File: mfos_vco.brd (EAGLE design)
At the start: 100 x 81.5 mm, 60 parts, among them IC1 TL072P, IC2 TL072P, IC3 TL072P, T1 2N3904, T2 2N3904, U1 POWER, U2 2N5457

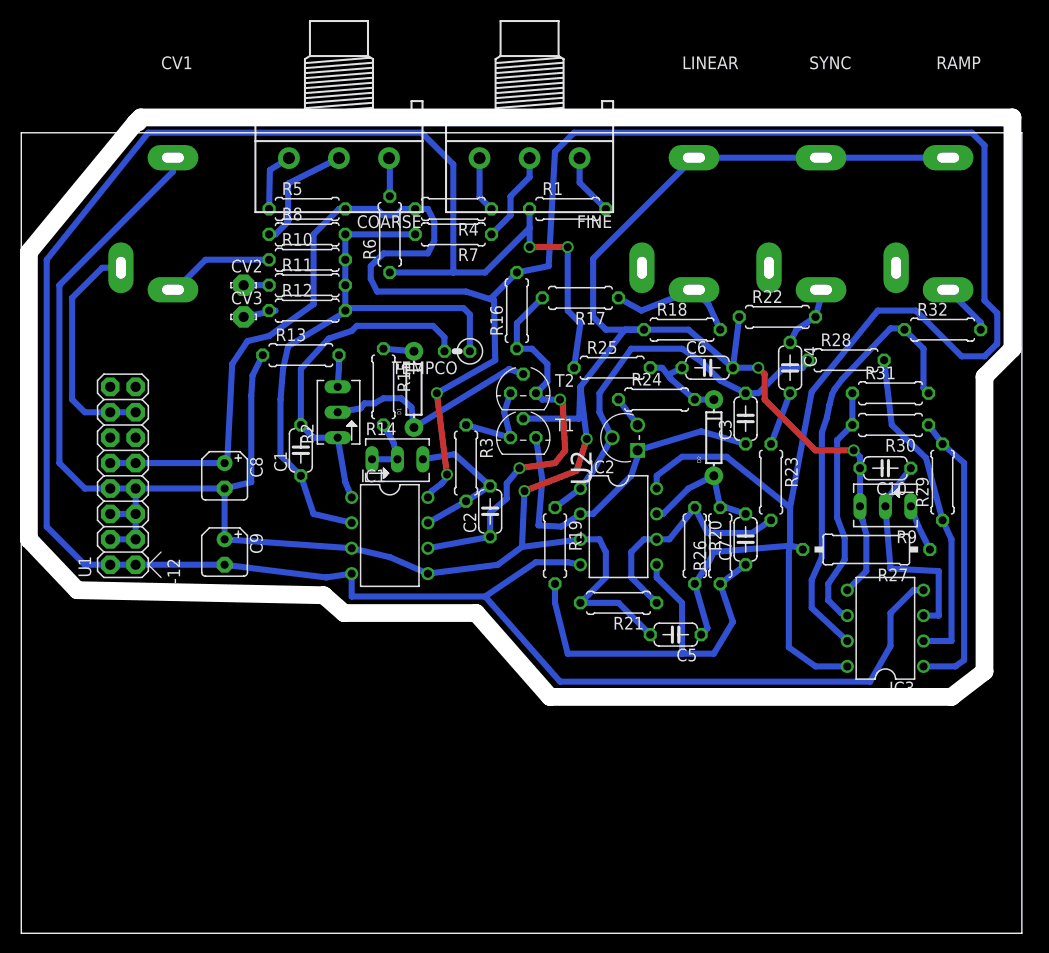
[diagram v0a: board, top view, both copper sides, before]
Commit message: ready to try lm394
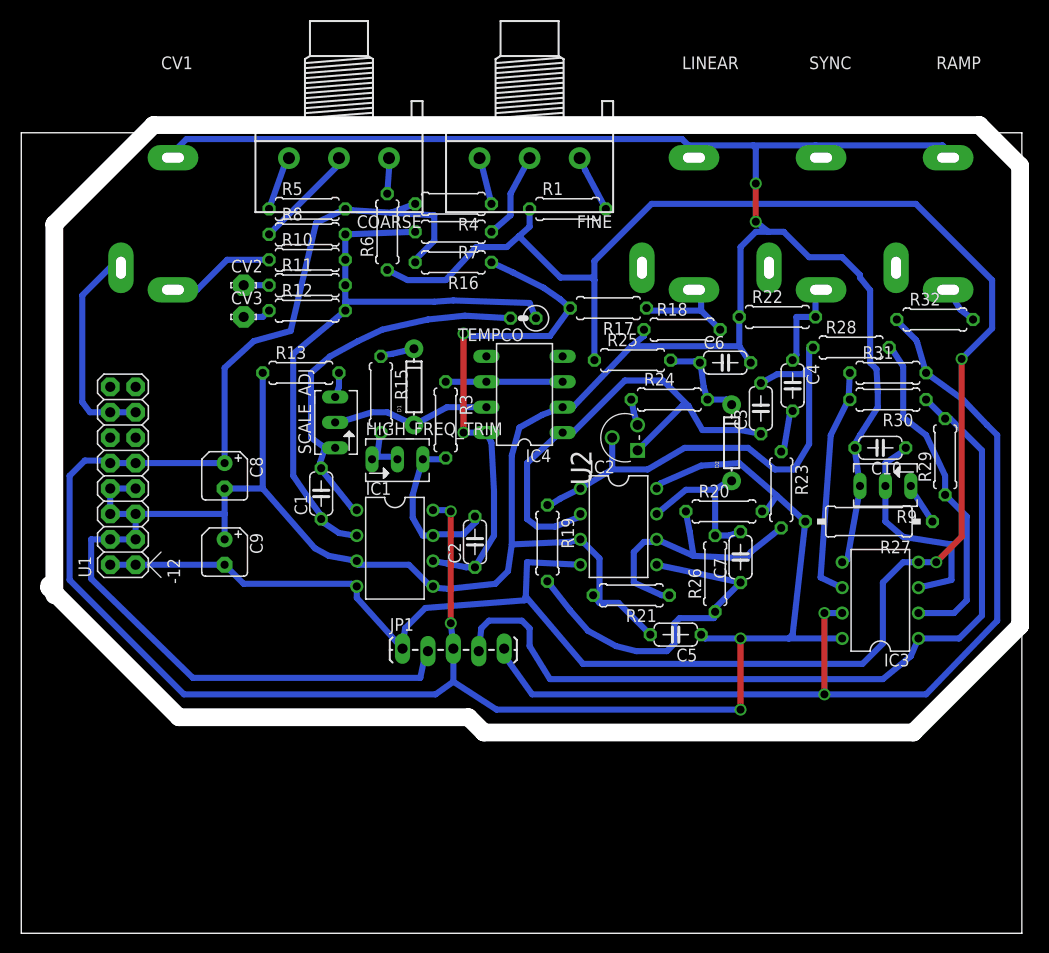
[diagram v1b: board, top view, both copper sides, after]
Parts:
- removed R2: 100R, pot:B64Y
- removed T1, T2: 2N3904, transistor:TO92
- added IC4: LM394N, synthdiy:DIL08
- added JP1: (no value), SparkFun-Connectors:1X05_LOCK_LONGPADS
- added SCALE_ADJ: 100R, pot:B64Y
- moved R16 7.98 mm to (43.2, 67.1), turned to 180 degrees
- moved TEMPCO 7.38 mm to (50.2, 61.5)
- moved R3 4.77 mm to (42.4, 51.3)
- moved C1 4.77 mm to (30.0, 43.9)
- moved R20 4.50 mm to (70.2, 42.2), turned to 0 degrees
- moved C2 3.41 mm to (45.3, 39.1)
- moved R17 2.97 mm to (58.7, 62.5)
- moved IC3 2.84 mm to (85.9, 33.3)
- moved R26 2.84 mm to (69.3, 35.9)
- moved R27 2.81 mm to (84.7, 41.1)
- moved R30 2.55 mm to (86.6, 53.3)
- moved R29 2.55 mm to (92.3, 47.6)
- moved R25 2.17 mm to (61.1, 57.3)
- moved C10 2.09 mm to (85.9, 48.5)
- moved R31 2.05 mm to (86.6, 56.0)
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- renumbered R14 to HIGH_FREQ_TRIM
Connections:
- net +12V: now also JP1.3
- net -12V: now also JP1.1
- net GND: now also IC4.2, JP1.2; no longer T1.2
- net N$12: now also IC4.3, IC4.6; no longer T1.3, T2.3
- net N$13: now also IC4.8; no longer T2.1
- net N$23: now also IC4.1; no longer T1.1
- net N$33: now also JP1.4
- net N$35: now also JP1.5
- net N$7: now also SCALE_ADJ.A; no longer R2.A
- net N$8: now also IC4.7, SCALE_ADJ.S; no longer R2.S, T2.2
- net N$9: now also SCALE_ADJ.E; no longer R2.E
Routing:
- net GND: track 274.4 -> 332.1 mm, vias 4 -> 2
- net +12V: track 277.0 -> 220.4 mm, vias 2 -> 4
- net N$35: track 44.2 -> 99.2 mm, vias 0 -> 2
- net N$33: track 29.2 -> 83.9 mm
- net N$23: track 34.0 -> 48.3 mm
- net N$13: track 40.7 -> 51.8 mm
- net -12V: track 233.9 -> 222.9 mm
- net N$21: track 40.0 -> 48.8 mm
- net N$22: track 42.6 -> 35.2 mm
- net N$8: track 22.8 -> 16.0 mm
- net N$9: track 33.9 -> 38.3 mm
- net N$26: track 24.1 -> 28.2 mm
- net N$10: track 59.7 -> 62.9 mm
- net N$30: track 12.9 -> 15.8 mm
- net N$25: track 6.50 -> 9.29 mm
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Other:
- board size 100 x 81.5 mm -> 100 x 80.8 mm
